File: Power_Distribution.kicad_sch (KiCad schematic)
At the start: 23 parts, among them IC1 TLV74033PDBVR, J7 CarPowerConnector, Q1 PBSS4330X,135, Q3 SI7149ADP-T1-GE3, U2 RI3-1205S

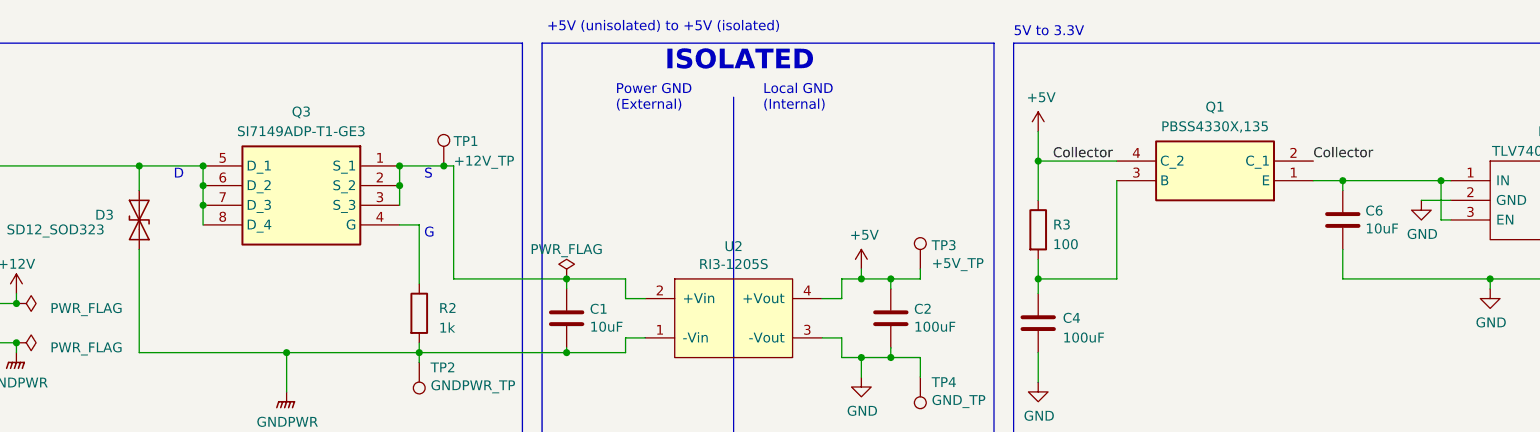
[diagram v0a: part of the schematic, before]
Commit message: changed BJT and PMOSFET symbols to standard schematic symbols
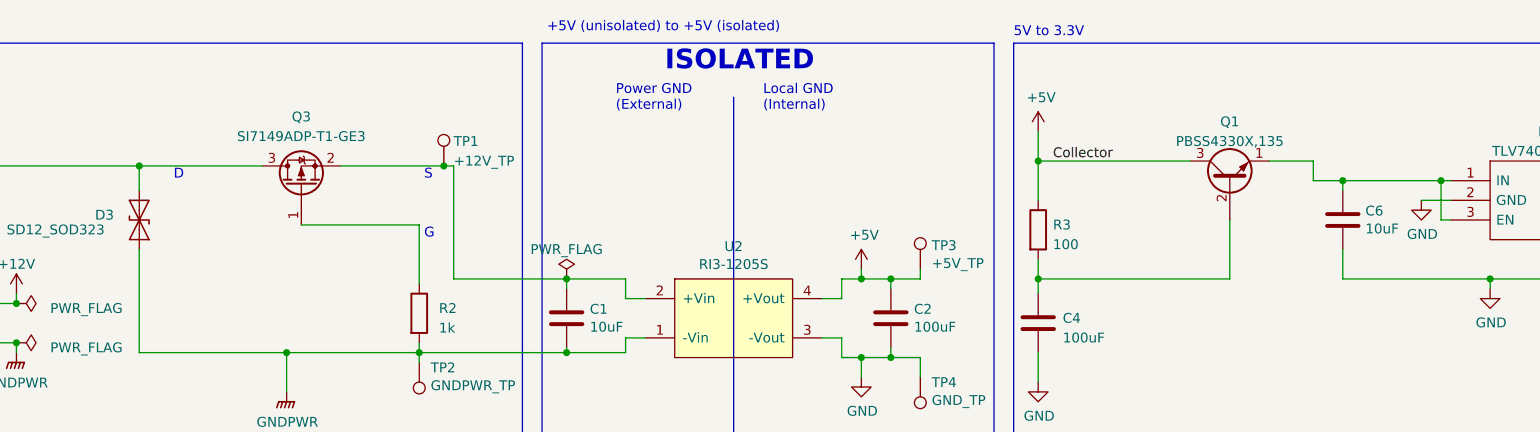
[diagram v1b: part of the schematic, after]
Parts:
- Q1: footprint PBSS4330X135 -> Package_TO_SOT_THT:TO-39-3; symbol UTSVT_LeaderSOM:PBSS4330X,135 -> Transistor_BJT:2N2219
- Q3: footprint POWERPAKSO-8 -> Package_TO_SOT_SMD:SOT-23; symbol UTSVT_LeaderSOM:SI7149ADP-T1-GE3 -> Transistor_FET:AO3401A
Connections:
- net +12V: now also Q3.3 (D); no longer Q3.5 (D_1), Q3.6 (D_2), Q3.7 (D_3), Q3.8 (D_4)
- net +5V: now also Q1.3 (C); no longer Q1.2 (C_1), Q1.4 (C_2)
- net at R2.1: now also Q3.1 (G); no longer Q3.4 (G)
- net at C4.1, R3.2: now also Q1.2 (B); no longer Q1.3 (B)
- net at C1.1, Q3.2 (S), TP1.1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: no longer Q3.1 (S_1), Q3.3 (S_3)
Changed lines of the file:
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@@
   (junction (at 102.87 60.325) (diameter 0) (color 0 0 0 0)
   )
-  (junction (at 74.93 41.275) (diameter 0) (color 0 0 0 0)
-  )
   (junction (at 121.92 50.8) (diameter 0) (color 0 0 0 0)
   )
@@
   (junction (at 182.88 50.8) (diameter 0) (color 0 0 0 0)
   )
-  (junction (at 74.93 36.195) (diameter 0) (color 0 0 0 0)
-  )
   (junction (at 41.91 99.06) (diameter 0) (color 0 0 0 0)
   )
-  (junction (at 74.93 38.735) (diameter 0) (color 0 0 0 0)
-  )
   (junction (at 66.675 36.195) (diameter 0) (color 0 0 0 0)
   )
@@
   (junction (at 62.865 99.06) (diameter 0) (color 0 0 0 0)
   )
-  (junction (at 100.33 36.195) (diameter 0) (color 0 0 0 0)
-  )
   (junction (at 121.92 60.325) (diameter 0) (color 0 0 0 0)
   )
-  (junction (at 100.33 38.735) (diameter 0) (color 0 0 0 0)
-  )
   (junction (at 82.55 99.06) (diameter 0) (color 0 0 0 0)
   )
@@
     (stroke (width 0) (type default))
   )
-  (wire (pts (xy 66.675 36.195) (xy 74.93 36.195))
+  (wire (pts (xy 207.645 43.18) (xy 207.645 50.8))
+    (stroke (width 0) (type default))
+  )
+  (wire (pts (xy 66.675 36.195) (xy 82.55 36.195))
     (stroke (width 0) (type default))
   )
@@
     (stroke (width 0) (type default))
   )
-  (wire (pts (xy 182.88 35.56) (xy 193.04 35.56))
-    (stroke (width 0) (type default))
-  )
   (wire (pts (xy 182.88 35.56) (xy 182.88 40.64))
     (stroke (width 0) (type default))
@@
     (stroke (width 0) (type default))
   )
+  (wire (pts (xy 182.88 35.56) (xy 202.565 35.56))
+    (stroke (width 0) (type default))
+  )
   (wire (pts (xy 236.22 43.18) (xy 234.95 43.18))
     (stroke (width 0) (type default))
@@
     (stroke (width 0) (type default))
   )
-  (wire (pts (xy 100.33 38.735) (xy 100.33 41.275))
-    (stroke (width 0) (type default))
-  )
   (wire (pts (xy 241.3 50.8) (xy 241.3 52.07))
     (stroke (width 0) (type default))
@@
     (stroke (width 0) (type default))
   )
+  (wire (pts (xy 92.71 36.195) (xy 106.045 36.195))
+    (stroke (width 0) (type default))
+  )
   (wire (pts (xy 167.64 49.53) (xy 167.64 50.8))
     (stroke (width 0) (type default))
   )
-  (wire (pts (xy 102.87 43.815) (xy 100.33 43.815))
+  (wire (pts (xy 87.63 43.815) (xy 102.87 43.815))
     (stroke (width 0) (type default))
   )
@@
     (stroke (width 0) (type default))
   )
-  (wire (pts (xy 193.04 38.1) (xy 193.04 50.8))
-    (stroke (width 0) (type default))
-  )
   (wire (pts (xy 182.88 48.26) (xy 182.88 50.8))
     (stroke (width 0) (type default))
   )
-  (wire (pts (xy 193.04 50.8) (xy 182.88 50.8))
+  (wire (pts (xy 207.645 50.8) (xy 182.88 50.8))
     (stroke (width 0) (type default))
   )
@@
     (stroke (width 0) (type default))
   )
-  (wire (pts (xy 74.93 38.735) (xy 74.93 41.275))
-    (stroke (width 0) (type default))
-  )
   (wire (pts (xy 129.54 53.34) (xy 132.08 53.34))
     (stroke (width 0) (type default))
@@
     (stroke (width 0) (type default))
   )
-  (wire (pts (xy 74.93 36.195) (xy 74.93 38.735))
-    (stroke (width 0) (type default))
-  )
   (polyline (pts (xy 143.51 27.305) (xy 143.51 71.12))
     (stroke (width 0) (type default))
@@
     (stroke (width 0) (type default))
   )
+  (wire (pts (xy 218.44 35.56) (xy 218.44 38.1))
+    (stroke (width 0) (type default))
+  )
   (wire (pts (xy 163.83 60.96) (xy 160.02 60.96))
     (stroke (width 0) (type default))
@@
     (stroke (width 0) (type default))
   )
-  (wire (pts (xy 74.93 41.275) (xy 74.93 43.815))
-    (stroke (width 0) (type default))
-  )
   (wire (pts (xy 182.88 31.75) (xy 182.88 35.56))
     (stroke (width 0) (type default))
@@
     (stroke (width 0) (type default))
   )
+  (wire (pts (xy 212.725 35.56) (xy 218.44 35.56))
+    (stroke (width 0) (type default))
+  )
   (wire (pts (xy 222.25 38.1) (xy 222.25 39.37))
     (stroke (width 0) (type default))
@@
     (stroke (width 0) (type default))
   )
-  (wire (pts (xy 100.33 36.195) (xy 100.33 38.735))
-    (stroke (width 0) (type default))
-  )
   (wire (pts (xy 154.94 58.42) (xy 157.48 58.42))
     (stroke (width 0) (type default))
@@
   )
   (wire (pts (xy 85.09 99.06) (xy 82.55 99.06))
-    (stroke (width 0) (type default))
-  )
-  (wire (pts (xy 100.33 36.195) (xy 106.045 36.195))
     (stroke (width 0) (type default))
   )
@@
   )
   (text "G\n" (at 103.505 45.72 0)
-    (effects (font (size 1.27 1.27)) (justify left bottom))
-  )
-  (label "Collector" (at 218.44 35.56 0) (fields_autoplaced)
     (effects (font (size 1.27 1.27)) (justify left bottom))
   )
@@
     )
   )
-  (symbol (lib_id "UTSVT_LeaderSOM:SI7149ADP-T1-GE3") (at 100.33 36.195 0) (mirror y) (unit 1)
-    (in_bom yes) (on_board yes) (dnp no)
-    (property "Reference" "Q3" (at 87.63 29.21 0)
-      (effects (font (size 1.27 1.27)))
-    )
-    (property "Value" "SI7149ADP-T1-GE3" (at 87.63 31.75 0)
-      (effects (font (size 1.27 1.27)))
-    )
-    (property "Footprint" "POWERPAKSO-8" (at 78.74 131.115 0)
+  (symbol (lib_id "Transistor_FET:AO3401A") (at 87.63 38.735 90) (unit 1)
+    (in_bom yes) (on_board yes) (dnp no)
+    (property "Reference" "Q3" (at 87.63 29.845 90)
+      (effects (font (size 1.27 1.27)))
+    )
+    (property "Value" "SI7149ADP-T1-GE3" (at 87.63 32.385 90)
+      (effects (font (size 1.27 1.27)))
+    )
+    (property "Footprint" "Package_TO_SOT_SMD:SOT-23" (at 89.535 33.655 0)
+      (effects (font (size 1.27 1.27) italic) (justify left) hide)
+    )
+    (property "Datasheet" "http://www.aosmd.com/pdfs/datasheet/AO3401A.pdf" (at 87.63 38.735 0)
+      (effects (font (size 1.27 1.27)) (justify left) hide)
+    )
+    (property "Height" "" (at 482.55 17.145 0)
       (effects (font (size 1.27 1.27)) (justify left top) hide)
     )
-    (property "Datasheet" "https://www.vishay.com/docs/62839/si7149adp.pdf" (at 78.74 231.115 0)
+    (property "Mouser Part Number" "78-SI7149ADP-T1-GE3" (at 582.55 17.145 0)
       (effects (font (size 1.27 1.27)) (justify left top) hide)
     )
-    (property "Height" "" (at 78.74 431.115 0)
+    (property "Mouser Price/Stock" "https://www.mouser.co.uk/ProductDetail/Vishay-Semiconductors/SI7149ADP-T1-GE3?qs=vgn07B5hXauIZBHl%2Fj5hoQ%3D%3D" (at 682.55 17.145 0)
       (effects (font (size 1.27 1.27)) (justify left top) hide)
     )
-    (property "Mouser Part Number" "78-SI7149ADP-T1-GE3" (at 78.74 531.115 0)
+    (property "Manufacturer_Name" "Vishay" (at 782.55 17.145 0)
       (effects (font (size 1.27 1.27)) (justify left top) hide)
     )
-    (property "Mouser Price/Stock" "https://www.mouser.co.uk/ProductDetail/Vishay-Semiconductors/SI7149ADP-T1-GE3?qs=vgn07B5hXauIZBHl%2Fj5hoQ%3D%3D" (at 78.74 631.115 0)
-      (effects (font (size 1.27 1.27)) (justify left top) hide)
-    )
-    (property "Manufacturer_Name" "Vishay" (at 78.74 731.115 0)
-      (effects (font (size 1.27 1.27)) (justify left top) hide)
-    )
-    (property "Manufacturer_Part_Number" "SI7149ADP-T1-GE3" (at 78.74 831.115 0)
+    (property "Manufacturer_Part_Number" "SI7149ADP-T1-GE3" (at 882.55 17.145 0)
       (effects (font (size 1.27 1.27)) (justify left top) hide)
     )
@@
     (pin "2")
     (pin "3")
-    (pin "4")
-    (pin "5")
-    (pin "6")
-    (pin "7")
-    (pin "8")
     (instances
       (project "LeaderSOM"
@@
     )
   )
-  (symbol (lib_id "UTSVT_LeaderSOM:PBSS4330X,135") (at 218.44 38.1 180) (unit 1)
+  (symbol (lib_id "Transistor_BJT:2N2219") (at 207.645 38.1 90) (unit 1)
     (in_bom yes) (on_board yes) (dnp no) (fields_autoplaced)
-    (property "Reference" "Q1" (at 205.74 28.575 0)
-      (effects (font (size 1.27 1.27)))
-    )
-    (property "Value" "PBSS4330X,135" (at 205.74 31.115 0)
-      (effects (font (size 1.27 1.27)))
-    )
-    (property "Footprint" "PBSS4330X135" (at 196.85 -56.82 0)
+    (property "Reference" "Q1" (at 207.645 30.48 90)
+      (effects (font (size 1.27 1.27)))
+    )
+    (property "Value" "PBSS4330X,135" (at 207.645 33.02 90)
+      (effects (font (size 1.27 1.27)))
+    )
+    (property "Footprint" "Package_TO_SOT_THT:TO-39-3" (at 209.55 33.02 0)
+      (effects (font (size 1.27 1.27) italic) (justify left) hide)
+    )
+    (property "Datasheet" "http://www.onsemi.com/pub_link/Collateral/2N2219-D.PDF" (at 207.645 38.1 0)
+      (effects (font (size 1.27 1.27)) (justify left) hide)
+    )
+    (property "Height" "1.6" (at 602.565 16.51 0)
       (effects (font (size 1.27 1.27)) (justify left top) hide)
     )
-    (property "Datasheet" "https://assets.nexperia.com/documents/data-sheet/PBSS4330X.pdf" (at 196.85 -156.82 0)
+    (property "Mouser Part Number" "771-PBSS4330X135" (at 702.565 16.51 0)
       (effects (font (size 1.27 1.27)) (justify left top) hide)
     )
-    (property "Height" "1.6" (at 196.85 -356.82 0)
+    (property "Mouser Price/Stock" "https://www.mouser.co.uk/ProductDetail/Nexperia/PBSS4330X135?qs=LOCUfHb8d9vXgka%252BQXAieA%3D%3D" (at 802.565 16.51 0)
       (effects (font (size 1.27 1.27)) (justify left top) hide)
     )
-    (property "Mouser Part Number" "771-PBSS4330X135" (at 196.85 -456.82 0)
+    (property "Manufacturer_Name" "Nexperia" (at 902.565 16.51 0)
       (effects (font (size 1.27 1.27)) (justify left top) hide)
     )
-    (property "Mouser Price/Stock" "https://www.mouser.co.uk/ProductDetail/Nexperia/PBSS4330X135?qs=LOCUfHb8d9vXgka%252BQXAieA%3D%3D" (at 196.85 -556.82 0)
-      (effects (font (size 1.27 1.27)) (justify left top) hide)
-    )
-    (property "Manufacturer_Name" "Nexperia" (at 196.85 -656.82 0)
-      (effects (font (size 1.27 1.27)) (justify left top) hide)
-    )
-    (property "Manufacturer_Part_Number" "PBSS4330X,135" (at 196.85 -756.82 0)
+    (property "Manufacturer_Part_Number" "PBSS4330X,135" (at 1002.565 16.51 0)
       (effects (font (size 1.27 1.27)) (justify left top) hide)
     )
@@
     (pin "2")
     (pin "3")
-    (pin "4")
-    (instances
-      (project "LeaderSOM"
+    (instances
+      (project "LeaderSOM"

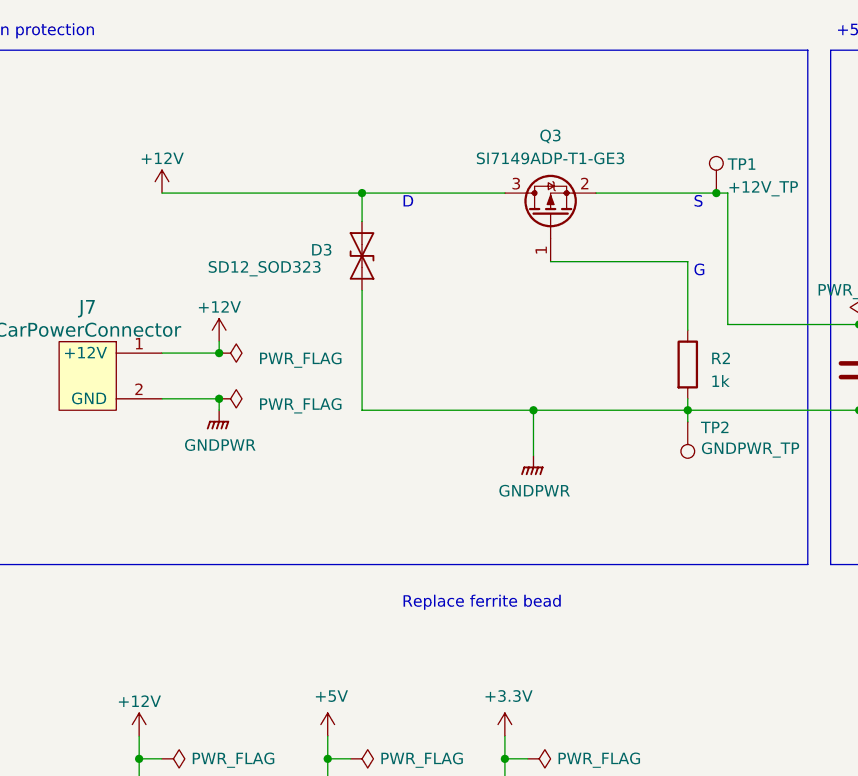
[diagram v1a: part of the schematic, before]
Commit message: Added power distribution ferrite bead
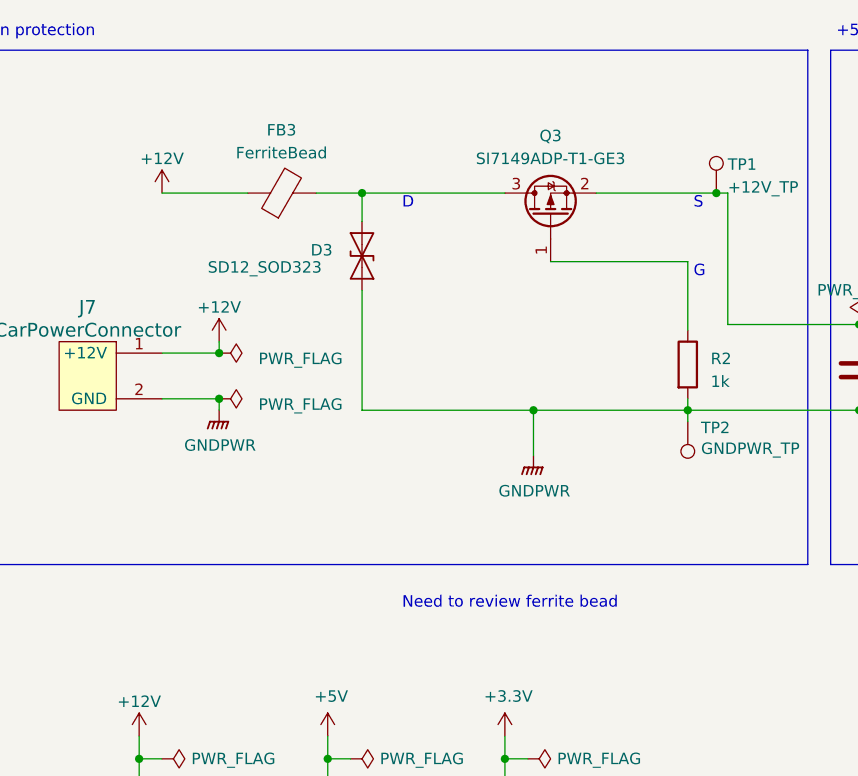
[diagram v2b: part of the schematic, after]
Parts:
- added FB3: FerriteBead, Inductor_SMD:L_0805_2012Metric, symbol Device:FerriteBead
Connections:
- net +12V: now also FB3.1; no longer D3.2 (A2), Q3.3 (D)
- new net: D3.2 (A2), FB3.2, Q3.3 (D)
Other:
- note added: "Need to review ferrite bead"
- note removed: "Replace ferrite bead"
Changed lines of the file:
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@@
+    (stroke (width 0) (type default))
+  )
+  (wire (pts (xy 61.595 36.195) (xy 66.675 36.195))
     (stroke (width 0) (type default))
   )
@@
     (stroke (width 0) (type default))
   )
-  (wire (pts (xy 44.45 36.195) (xy 66.675 36.195))
+  (wire (pts (xy 44.45 36.195) (xy 53.975 36.195))
     (stroke (width 0) (type default))
   )
@@
     (fill (type none))
   )
-  (text "Replace ferrite bead" (at 71.12 82.55 0)
+  (text "Need to review ferrite bead" (at 71.12 82.55 0)
     (effects (font (size 1.27 1.27)) (justify left bottom))
   )
@@
         )
       )
+    )
+  )
+  (symbol (lib_id "Device:FerriteBead") (at 57.785 36.195 90) (unit 1)
+    (in_bom yes) (on_board yes) (dnp no) (fields_autoplaced)
+    (property "Reference" "FB3" (at 57.7342 29.21 90)
+      (effects (font (size 1.27 1.27)))
+    )
+    (property "Value" "FerriteBead" (at 57.7342 31.75 90)
+      (effects (font (size 1.27 1.27)))
+    )
+    (property "Footprint" "Inductor_SMD:L_0805_2012Metric" (at 57.785 37.973 90)
+      (effects (font (size 1.27 1.27)) hide)
+    )
+    (property "Datasheet" "https://www.we-online.com/components/products/datasheet/742792017.pdf" (at 57.785 36.195 0)
+      (effects (font (size 1.27 1.27)) hide)
+    )
+    (pin "1")
+    (pin "2")
+    (instances
+      (project "LeaderSOM"
+        (path "/192d0c36-944e-4927-949b-263b8c85a7ca/07cef2e6-f2f4-4f04-bcaf-7b98b53ab0fe"
+          (reference "FB3") (unit 1)
+        )
+      )

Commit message: Updated datasheets
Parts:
- C4: footprint (none) -> Capacitor_SMD:C_0805_2012Metric
- J7: footprint (none) -> UTSVT_Connectors:Molex_MicroFit3.0_1x2xP3.00mm_PolarizingPeg_Vertical
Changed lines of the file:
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@@
       (effects (font (size 1.27 1.27)) (justify left))
     )
-    (property "Footprint" "" (at 183.8452 60.325 0)
+    (property "Footprint" "Capacitor_SMD:C_0805_2012Metric" (at 183.8452 60.325 0)
       (effects (font (size 1.27 1.27)) hide)
     )
@@
       (effects (font (size 1.524 1.524)))
     )
-    (property "Footprint" "" (at 36.83 56.515 0)
+    (property "Footprint" "UTSVT_Connectors:Molex_MicroFit3.0_1x2xP3.00mm_PolarizingPeg_Vertical" (at 36.83 56.515 0)
       (effects (font (size 1.524 1.524)) hide)
     )
-    (property "Datasheet" "" (at 36.83 56.515 0)
+    (property "Datasheet" "https://www.mouser.com/ProductDetail/Molex/43650-0244?qs=XoD1gVtqLQuEe6RJ38AzJQ%3D%3D" (at 36.83 56.515 0)
       (effects (font (size 1.524 1.524)) hide)
     )
